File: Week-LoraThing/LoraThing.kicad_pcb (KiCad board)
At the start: 2 copper layers, 27 x 43 mm, 33 parts, among them J1 Conn_01x07_Male, J2 Conn_01x07_Male, J3 Conn_01x01_Female, U1 AP7333-33SRG-7, U2 RFM95W-868S2

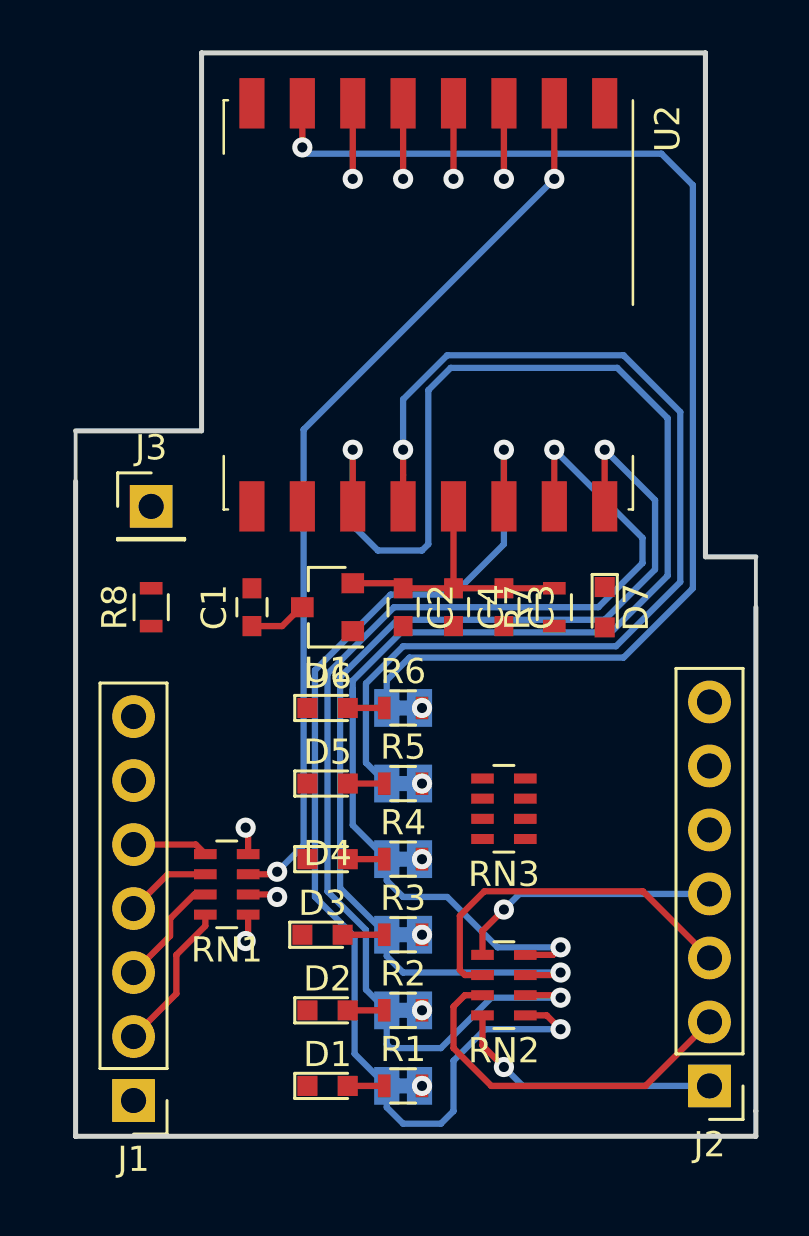
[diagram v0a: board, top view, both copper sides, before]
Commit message: Resyn forgot to save first (again)
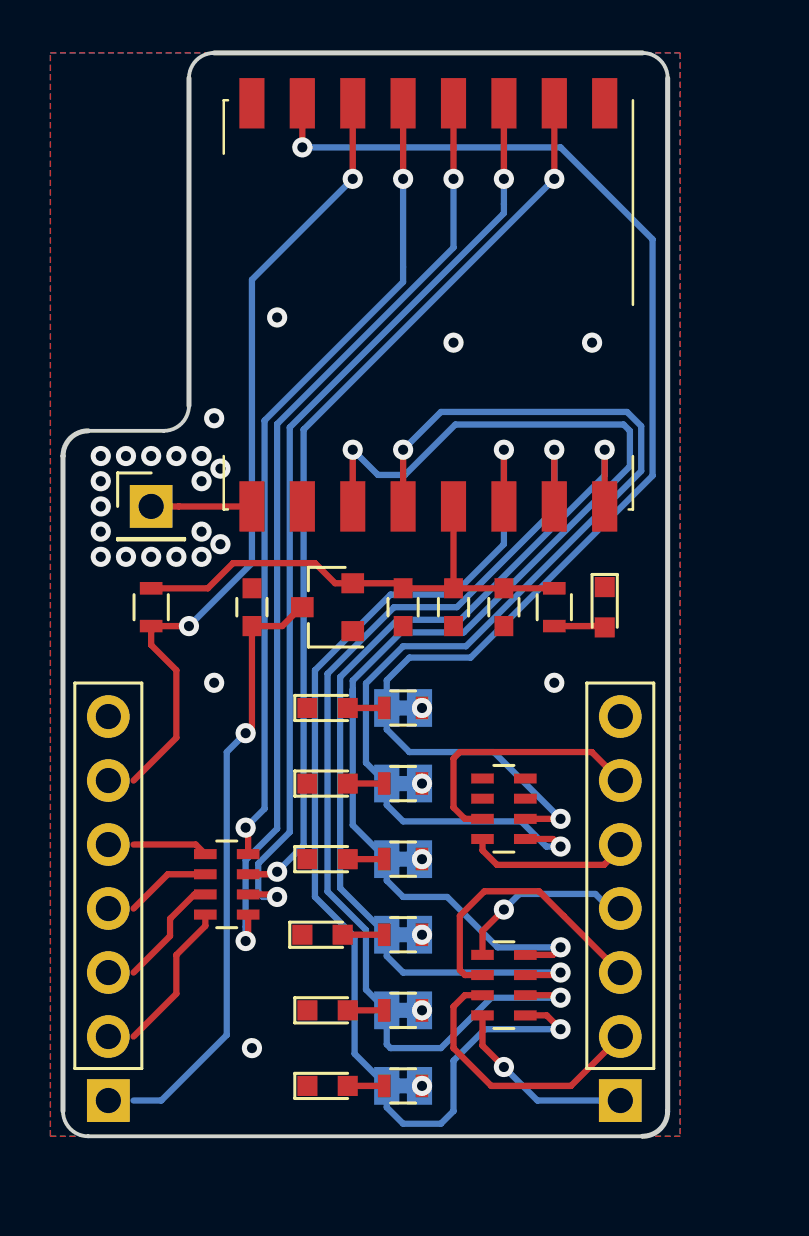
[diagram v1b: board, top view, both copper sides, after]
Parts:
- moved J2 3.59 mm to (133.6, 68.6)
- moved J1 1.00 mm to (113.3, 68.6)
- renumbered JP3 to eJP3
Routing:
- net /SPI_SCK: track 4.09 -> 37.8 mm
- net /SPI_MOSI: track 4.19 -> 37.4 mm
- net /RESET: track 3.00 -> 32.2 mm, vias 1 -> 2
- net /SPI_CS: track 4.09 -> 32.4 mm
- net VCC: track 2.31 -> 23.7 mm, vias 0 -> 1
- net /GPIO4: track 64.3 -> 48.8 mm
- net /EXT_GPIO6: track 0.00 -> 10.5 mm
- net +3V3: track 11.3 -> 20.1 mm
- net /EXT_GPIO5: track 0.00 -> 6.59 mm
- net /GPIO2: track 47.4 -> 41.2 mm
- net /GPIO3: track 42.5 -> 37.5 mm
- net /GPIO6: track 48.5 -> 52.6 mm, vias 1 -> 2
- net /ANTENNA: track 0.00 -> 4.00 mm
- net /EXT_GPIO2: track 14.8 -> 11.0 mm
- net /EXT_GPIO4: track 10.6 -> 7.27 mm
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- added copper zone on B.Cu, net GND
- added copper zone on F.Cu, net GND
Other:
- board size 27 x 43 mm -> 24 x 43 mm
